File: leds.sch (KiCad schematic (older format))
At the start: 32 parts

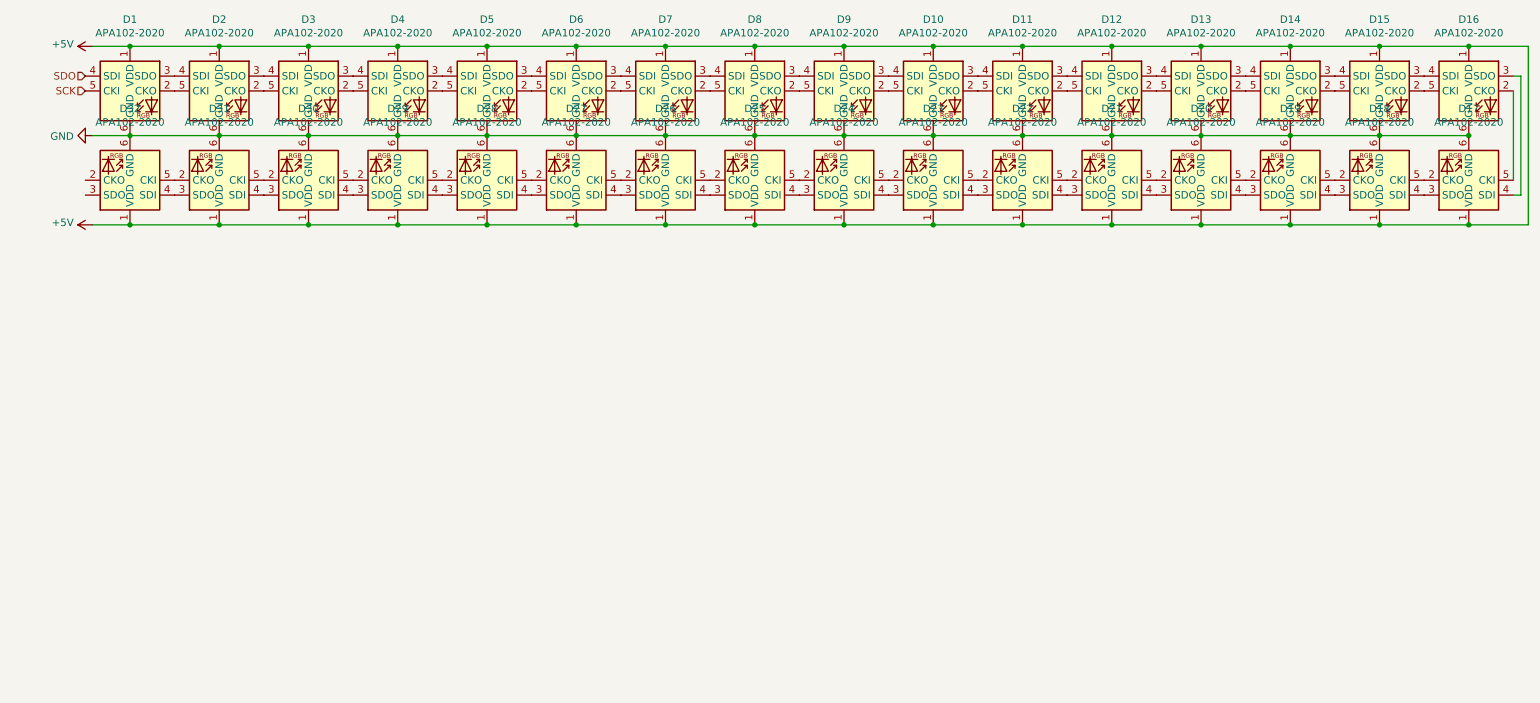
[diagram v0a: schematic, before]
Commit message: start working on spokes
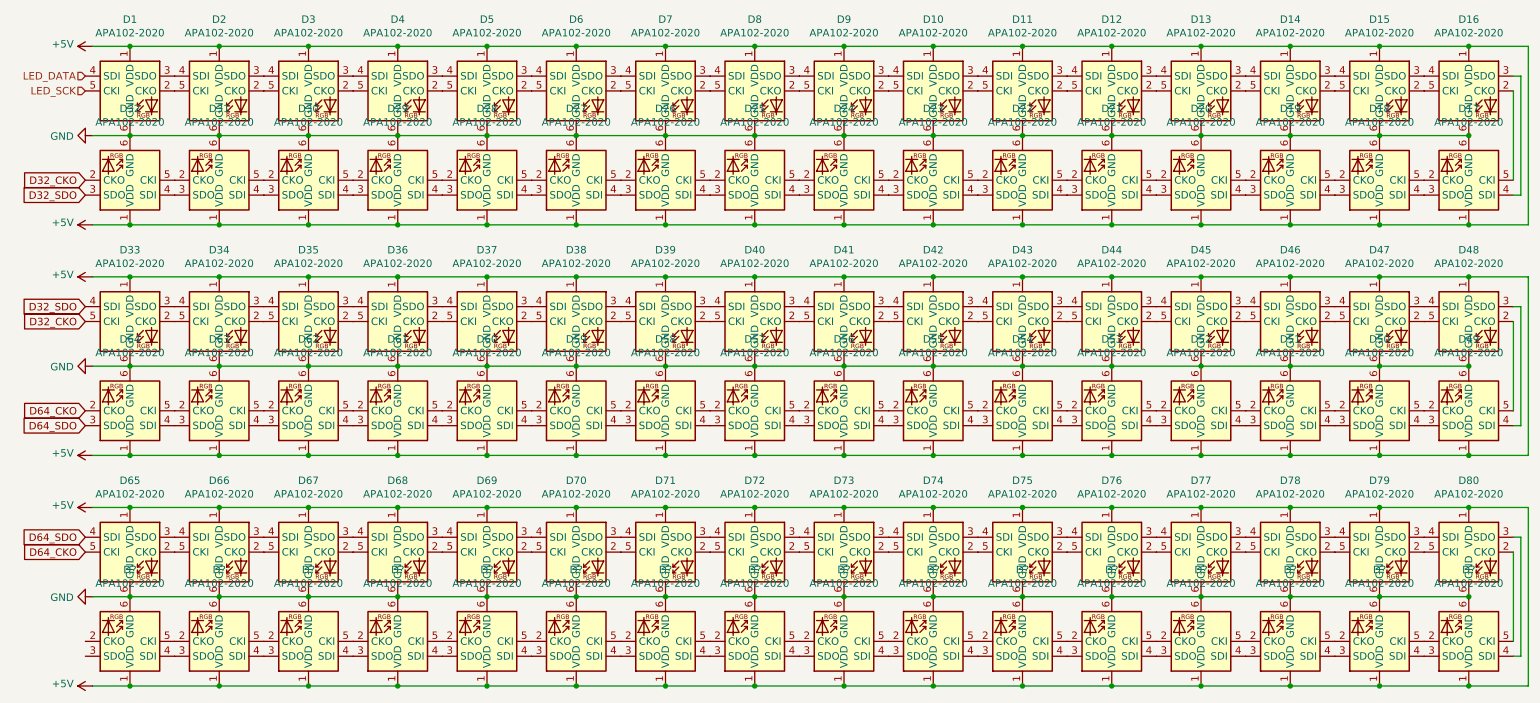
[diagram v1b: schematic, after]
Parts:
- added D33, D34, D35, D36, D37, D38, D39, D40, D41, D42, D43, D44, D45, D46, D47, D48, D49, D50, D51, D52, D53, D54, D55, D56, D57, D58, D59, D60, D61, D62, D63, D64, D65, D66, D67, D68, D69, D70, D71, D72, D73, D74, D75, D76, D77, D78, D79, D80, D? (x16): APA102-2020, LED_SMD:LED-APA102-2020_tightened_pads, symbol LED:APA102-2020
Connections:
- net +5V: now also D33.1 (VDD), D34.1 (VDD), D35.1 (VDD), D36.1 (VDD), D37.1 (VDD), D38.1 (VDD), D39.1 (VDD), D40.1 (VDD), D41.1 (VDD), D42.1 (VDD), D43.1 (VDD), D44.1 (VDD), D45.1 (VDD), D46.1 (VDD), D47.1 (VDD), D48.1 (VDD), D49.1 (VDD), D50.1 (VDD), D51.1 (VDD), D52.1 (VDD), D53.1 (VDD), D54.1 (VDD), D55.1 (VDD), D56.1 (VDD), D57.1 (VDD), D58.1 (VDD), D59.1 (VDD), D60.1 (VDD), D61.1 (VDD), D62.1 (VDD), D63.1 (VDD), D64.1 (VDD), D65.1 (VDD), D66.1 (VDD), D67.1 (VDD), D68.1 (VDD), D69.1 (VDD), D70.1 (VDD), D71.1 (VDD), D72.1 (VDD), D73.1 (VDD), D74.1 (VDD), D75.1 (VDD), D76.1 (VDD), D77.1 (VDD), D78.1 (VDD), D79.1 (VDD), D80.1 (VDD), D?.1 (VDD), D?.1 (VDD), D?.1 (VDD), D?.1 (VDD), D?.1 (VDD), D?.1 (VDD), D?.1 (VDD), D?.1 (VDD), D?.1 (VDD), D?.1 (VDD), D?.1 (VDD), D?.1 (VDD), D?.1 (VDD), D?.1 (VDD), D?.1 (VDD), D?.1 (VDD)
- net GND: now also D33.6 (GND), D34.6 (GND), D35.6 (GND), D36.6 (GND), D37.6 (GND), D38.6 (GND), D39.6 (GND), D40.6 (GND), D41.6 (GND), D42.6 (GND), D43.6 (GND), D44.6 (GND), D45.6 (GND), D46.6 (GND), D47.6 (GND), D48.6 (GND), D49.6 (GND), D50.6 (GND), D51.6 (GND), D52.6 (GND), D53.6 (GND), D54.6 (GND), D55.6 (GND), D56.6 (GND), D57.6 (GND), D58.6 (GND), D59.6 (GND), D60.6 (GND), D61.6 (GND), D62.6 (GND), D63.6 (GND), D64.6 (GND), D65.6 (GND), D66.6 (GND), D67.6 (GND), D68.6 (GND), D69.6 (GND), D70.6 (GND), D71.6 (GND), D72.6 (GND), D73.6 (GND), D74.6 (GND), D75.6 (GND), D76.6 (GND), D77.6 (GND), D78.6 (GND), D79.6 (GND), D80.6 (GND), D?.6 (GND), D?.6 (GND), D?.6 (GND), D?.6 (GND), D?.6 (GND), D?.6 (GND), D?.6 (GND), D?.6 (GND), D?.6 (GND), D?.6 (GND), D?.6 (GND), D?.6 (GND), D?.6 (GND), D?.6 (GND), D?.6 (GND), D?.6 (GND)
- net D32_CKO: now reaches D32.2 (CKO)
- net D32_CKO: now also D33.5 (CKI)
- net D32_SDO: now reaches D32.3 (SDO)
- net D32_SDO: now also D33.4 (SDI)
- net SCK renamed LED_SCK
- net SDO renamed LED_DATA
- new net: D48.2 (CKO), D49.5 (CKI)
- new net: D48.3 (SDO), D49.4 (SDI)
- new net: D47.3 (SDO), D48.4 (SDI)
- new net: D47.2 (CKO), D48.5 (CKI)
- new net: D46.3 (SDO), D47.4 (SDI)
- new net: D46.2 (CKO), D47.5 (CKI)
- new net: D45.3 (SDO), D46.4 (SDI)
- new net: D45.2 (CKO), D46.5 (CKI)
- new net: D44.3 (SDO), D45.4 (SDI)
- new net: D44.2 (CKO), D45.5 (CKI)
- new net: D43.3 (SDO), D44.4 (SDI)
- new net: D43.2 (CKO), D44.5 (CKI)
- new net: D42.3 (SDO), D43.4 (SDI)
- new net: D42.2 (CKO), D43.5 (CKI)
- new net: D41.3 (SDO), D42.4 (SDI)
- new net: D41.2 (CKO), D42.5 (CKI)
- new net: D40.3 (SDO), D41.4 (SDI)
- new net: D40.2 (CKO), D41.5 (CKI)
- new net: D39.3 (SDO), D40.4 (SDI)
- new net: D39.2 (CKO), D40.5 (CKI)
- new net: D38.3 (SDO), D39.4 (SDI)
- new net: D38.2 (CKO), D39.5 (CKI)
- new net: D37.3 (SDO), D38.4 (SDI)
- new net: D37.2 (CKO), D38.5 (CKI)
- new net: D36.3 (SDO), D37.4 (SDI)
- new net: D36.2 (CKO), D37.5 (CKI)
- new net: D35.3 (SDO), D36.4 (SDI)
- new net: D35.2 (CKO), D36.5 (CKI)
- new net: D34.3 (SDO), D35.4 (SDI)
- new net: D34.2 (CKO), D35.5 (CKI)
- new net: D33.3 (SDO), D34.4 (SDI)
- new net: D33.2 (CKO), D34.5 (CKI)
- new net: D49.2 (CKO), D50.5 (CKI)
- new net: D49.3 (SDO), D50.4 (SDI)
- new net: D50.2 (CKO), D51.5 (CKI)
- new net: D50.3 (SDO), D51.4 (SDI)
- new net: D51.2 (CKO), D52.5 (CKI)
- new net: D51.3 (SDO), D52.4 (SDI)
- new net: D52.2 (CKO), D53.5 (CKI)
- new net: D52.3 (SDO), D53.4 (SDI)
- new net: D53.2 (CKO), D54.5 (CKI)
- new net: D53.3 (SDO), D54.4 (SDI)
- new net: D54.2 (CKO), D55.5 (CKI)
- new net: D54.3 (SDO), D55.4 (SDI)
- new net: D55.2 (CKO), D56.5 (CKI)
- new net: D55.3 (SDO), D56.4 (SDI)
- new net: D56.2 (CKO), D57.5 (CKI)
- new net: D56.3 (SDO), D57.4 (SDI)
- new net: D57.2 (CKO), D58.5 (CKI)
- new net: D57.3 (SDO), D58.4 (SDI)
- new net: D58.2 (CKO), D59.5 (CKI)
- new net: D58.3 (SDO), D59.4 (SDI)
- new net: D59.2 (CKO), D60.5 (CKI)
- new net: D59.3 (SDO), D60.4 (SDI)
- new net: D60.2 (CKO), D61.5 (CKI)
- new net: D60.3 (SDO), D61.4 (SDI)
- new net: D61.2 (CKO), D62.5 (CKI)
- new net: D61.3 (SDO), D62.4 (SDI)
- new net: D62.2 (CKO), D63.5 (CKI)
- new net: D62.3 (SDO), D63.4 (SDI)
- new net: D63.2 (CKO), D64.5 (CKI)
- new net: D63.3 (SDO), D64.4 (SDI)
- new net: D80.2 (CKO), D?.5 (CKI)
- new net: D80.3 (SDO), D?.4 (SDI)
- new net: D79.3 (SDO), D80.4 (SDI)
- new net: D79.2 (CKO), D80.5 (CKI)
- new net: D78.3 (SDO), D79.4 (SDI)
- new net: D78.2 (CKO), D79.5 (CKI)
- new net: D77.3 (SDO), D78.4 (SDI)
- new net: D77.2 (CKO), D78.5 (CKI)
- new net: D76.3 (SDO), D77.4 (SDI)
- new net: D76.2 (CKO), D77.5 (CKI)
- new net: D75.3 (SDO), D76.4 (SDI)
- new net: D75.2 (CKO), D76.5 (CKI)
- new net: D74.3 (SDO), D75.4 (SDI)
- new net: D74.2 (CKO), D75.5 (CKI)
- new net: D73.3 (SDO), D74.4 (SDI)
- new net: D73.2 (CKO), D74.5 (CKI)
- new net: D72.3 (SDO), D73.4 (SDI)
- new net: D72.2 (CKO), D73.5 (CKI)
- new net: D71.3 (SDO), D72.4 (SDI)
- new net: D71.2 (CKO), D72.5 (CKI)
- new net: D70.3 (SDO), D71.4 (SDI)
- new net: D70.2 (CKO), D71.5 (CKI)
- new net: D69.3 (SDO), D70.4 (SDI)
- new net: D69.2 (CKO), D70.5 (CKI)
- new net: D68.3 (SDO), D69.4 (SDI)
- new net: D68.2 (CKO), D69.5 (CKI)
- new net: D67.3 (SDO), D68.4 (SDI)
- new net: D67.2 (CKO), D68.5 (CKI)
- new net: D66.3 (SDO), D67.4 (SDI)
- new net: D66.2 (CKO), D67.5 (CKI)
- new net: D65.3 (SDO), D66.4 (SDI)
- new net: D65.2 (CKO), D66.5 (CKI)
- new net: D?.2 (CKO), D?.5 (CKI) (x15)
- new net: D?.3 (SDO), D?.4 (SDI) (x15)
- new net D64_CKO: D64.2 (CKO), D65.5 (CKI)
- new net D64_SDO: D64.3 (SDO), D65.4 (SDI)
